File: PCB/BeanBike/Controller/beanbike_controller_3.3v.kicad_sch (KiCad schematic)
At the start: 11 parts

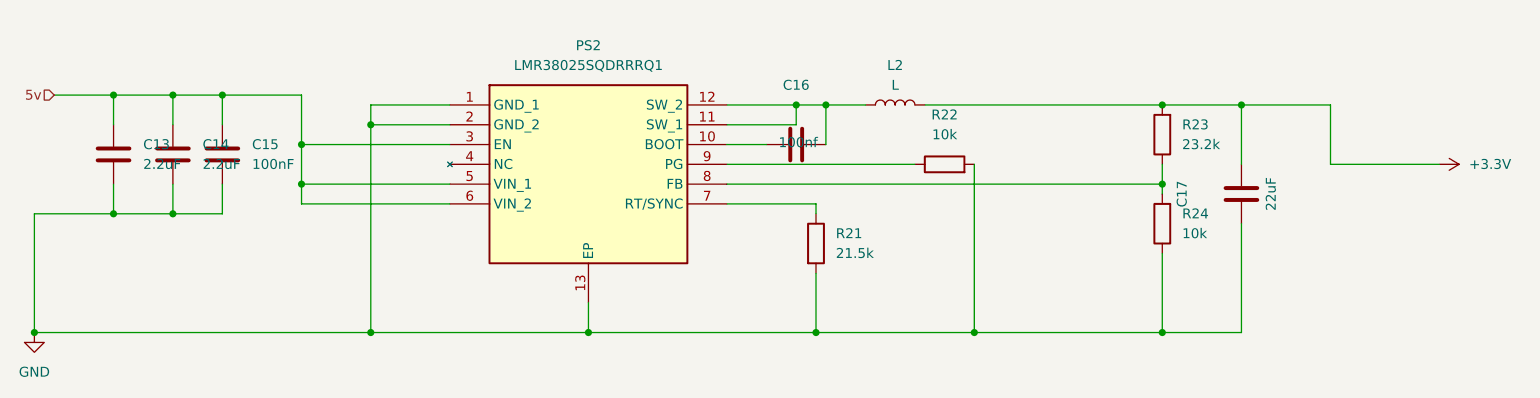
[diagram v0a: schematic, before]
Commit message: Forgot to commit
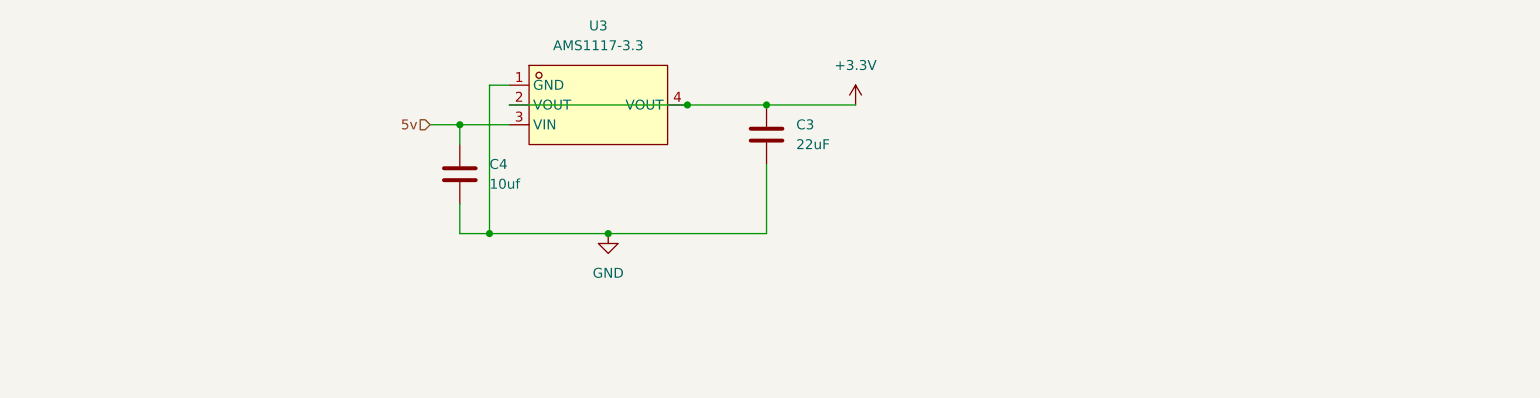
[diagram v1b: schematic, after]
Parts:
- removed C13, C14: 2.2uF, Capacitor_SMD:C_0201_0603Metric, symbol Device:C
- removed C15: 100nF, Capacitor_SMD:C_0201_0603Metric, symbol Device:C
- removed C16: 100nf, Capacitor_SMD:C_0201_0603Metric, symbol Device:C
- removed C17: 22uF, Capacitor_SMD:C_0603_1608Metric, symbol Device:C
- removed L2: L, easyeda2kicad:IND-SMD_L4.8-W4.5, symbol Device:L
- removed PS2: LMR38025SQDRRRQ1, LMR380:SON50P300X300X80-13N, symbol LMR38025SQDRRRQ1:LMR38025SQDRRRQ1
- removed R21: 21.5k, Resistor_SMD:R_0402_1005Metric, symbol Device:R
- removed R22, R24: 10k, Resistor_SMD:R_0603_1608Metric, symbol Device:R
- removed R23: 23.2k, Resistor_SMD:R_0402_1005Metric, symbol Device:R
- added C3: 22uF, symbol Device:C
- added C4: 10uf, symbol Device:C
- added U3: AMS1117-3.3, easyeda2kicad:SOT-223-3_L6.5-W3.4-P2.30-LS7.0-BR, symbol easyeda2kicad:AMS1117-3.3
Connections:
- net +3.3V: now also C3.1, U3.2 (VOUT), U3.4 (VOUT)
- net 5v: now also C4.1, U3.3 (VIN)
- net GND: now also C3.2, C4.2, U3.1 (GND)

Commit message: Footprints
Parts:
- C3: footprint (none) -> Capacitor_SMD:C_0201_0603Metric; LCSC (none) -> C59461
- C4: footprint (none) -> Capacitor_SMD:C_0402_1005Metric; LCSC (none) -> C15525
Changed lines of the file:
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@@
 			)
 		)
-		(property "Footprint" ""
+		(property "Footprint" "Capacitor_SMD:C_0402_1005Metric"
 			(at 126.6952 107.95 0)
 			(effects
@@
 		)
 		(property "Description" "Unpolarized capacitor"
+			(at 125.73 104.14 0)
+			(effects
+				(font
+					(size 1.27 1.27)
+				)
+				(hide yes)
+			)
+		)
+		(property "LCSC" "C15525"
 			(at 125.73 104.14 0)
 			(effects
@@
 			)
 		)
-		(property "Footprint" ""
+		(property "Footprint" "Capacitor_SMD:C_0201_0603Metric"
 			(at 166.0652 102.87 0)
 			(effects
@@
 			(at 165.1 99.06 0)
 			(effects
+				(font
+					(size 1.27 1.27)
+				)
+				(hide yes)
+			)
+		)
+		(property "LCSC" "C59461"
+			(at 165.1 99.06 0)
+			(effects
